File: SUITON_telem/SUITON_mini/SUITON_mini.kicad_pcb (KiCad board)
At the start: 2 copper layers, 81 parts, among them J3 USB_C_Receptacle_USB2.0_16P, Q2 AO3407A, Q3 BSS138, Q4 BSS138, Q5 BSS138, U1 W25Q128JVPIQ, U10 LSM6DSV320XTR, U11 USBLC6-2P6, U12 TPS1H200AQDGNRQ1, U13 AP2112K-3.3TRG1, U14 TPS1H200AQDGNRQ1, U2 TPS63070RNMR, U4 AP2112K-3.3TRG1, U5 STM32F405RGT6, U6 E22-900MM22S, U7 ISM330DHCXTR, U8 SAM-M10Q-00B, U9 BMP581, X1 ABM3B-8.000MHZ-10-1UT

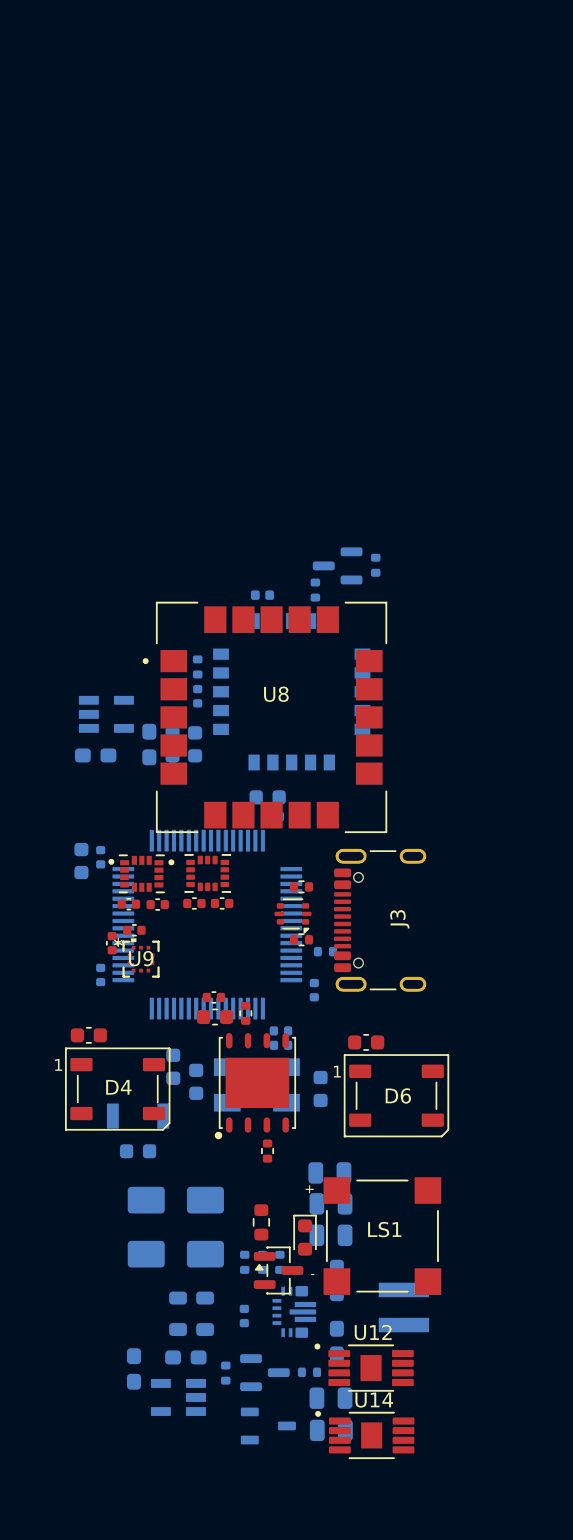
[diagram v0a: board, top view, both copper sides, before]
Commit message: Shape
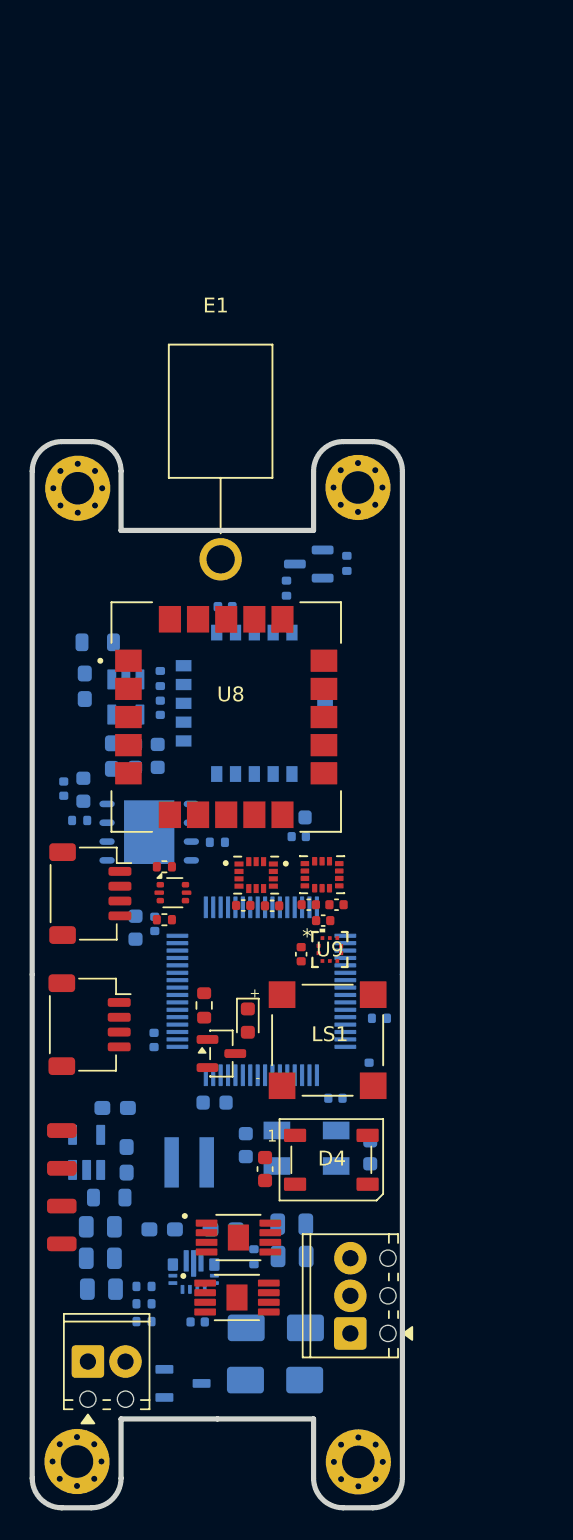
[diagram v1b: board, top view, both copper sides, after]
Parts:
- removed C21, C36: 100nF, Capacitor_SMD:C_0603_1608Metric
- removed C35: 1uF, Capacitor_SMD:C_0402_1005Metric
- removed D3, D7: SS34, Diode_SMD:D_SMA
- removed D6: WS2812B, LED_SMD:LED_WS2812B_PLCC4_5.0x5.0mm_P3.2mm
- removed J3: USB_C_Receptacle_USB2.0_16P, Connector_USB:USB_C_Receptacle_GCT_USB4105-xx-A_16P_TopMnt_Horizontal
- removed Q5: BSS138, Package_TO_SOT_SMD:SOT-23
- removed R2: 100kΩ, Resistor_SMD:R_0402_1005Metric
- removed S3: B3U-1000P, B3U-1000P:SW_B3U-1000P
- added D8: SS34, Diode_SMD:D_SMA, B.Cu at (145.4, 135.4)
- added D9: SS34, Diode_SMD:D_SMA, B.Cu at (145.5, 131.9)
- added E1: ANT-868-JJB-RA, ANT-868-JJB-RA:XDCR_ANT-868-JJB-RA, F.Cu at (141.8, 80.0)
- added H1: MountingHole_Pad, MountingHole:MountingHole_2.2mm_M2_Pad_Via, F.Cu at (132.1, 75.2)
- added H2: MountingHole_Pad, MountingHole:MountingHole_2.2mm_M2_Pad_Via, F.Cu at (151.1, 75.1)
- added H3: MountingHole_Pad, MountingHole:MountingHole_2.2mm_M2_Pad_Via, F.Cu at (132.1, 140.9)
- added H4: MountingHole_Pad, MountingHole:MountingHole_2.2mm_M2_Pad_Via, F.Cu at (151.1, 140.9)
- added J1: Conn_01x02_Pin, TerminalBlock_Phoenix:TerminalBlock_Phoenix_MPT-0,5-2-2.54_1x02_P2.54mm_Horizontal, F.Cu at (132.8, 134.2)
- added J2: Conn_01x04_Pin, Connector_JST:JST_SH_SM04B-SRSS-TB_1x04-1MP_P1.00mm_Horizontal, F.Cu at (133.0, 102.5)
- added J2: Conn_01x04_Pin, Connector_JST:JST_SH_SM04B-SRSS-TB_1x04-1MP_P1.00mm_Horizontal, F.Cu at (132.9, 111.4)
- added J5: Conn_01x03_Pin, TerminalBlock_Phoenix:TerminalBlock_Phoenix_MPT-0,5-3-2.54_1x03_P2.54mm_Horizontal, F.Cu at (150.5, 132.2)
- added J6: Conn_01x01_Pin, Connector_Wire:SolderWirePad_1x01_SMD_1x2mm, F.Cu at (131.1, 126.2)
- added J7: Conn_01x01_Pin, Connector_Wire:SolderWirePad_1x01_SMD_1x2mm, F.Cu at (131.1, 123.7)
- added J8: Conn_01x01_Pin, Connector_Wire:SolderWirePad_1x01_SMD_1x2mm, F.Cu at (131.1, 121.1)
- added J9: Conn_01x01_Pin, Connector_Wire:SolderWirePad_1x01_SMD_1x2mm, F.Cu at (131.1, 118.6)
- C22, C23, R30, R31, U1: moved to B.Cu
- moved FB2 45.7 mm to (133.5, 85.6), turned to 0 degrees
- moved R30 21.1 mm to (141.6, 99.1), turned to 180 degrees
- moved U1 18.4 mm to (136.9, 98.4), turned to 180 degrees
- moved C23 17.7 mm to (132.5, 95.5), turned to -90 degrees
- moved U4 17.7 mm to (132.7, 120.0), turned to 90 degrees
- moved C11 17.7 mm to (134.7, 117.0), turned to 0 degrees
- moved L3 17.5 mm to (139.7, 120.7), turned to 0 degrees
- moved C22 17.4 mm to (131.2, 95.5), turned to -90 degrees
- moved C8 17.3 mm to (133.7, 129.3), turned to 180 degrees
- moved R31 17.2 mm to (132.3, 97.6), turned to 0 degrees
- moved U14 16.1 mm to (143.0, 125.8)
- moved C7 16.0 mm to (133.7, 127.2), turned to 180 degrees
- moved C6 15.6 mm to (133.7, 125.0), turned to 180 degrees
- moved D4 15.2 mm to (149.2, 120.5)
- moved D5 15.2 mm to (143.6, 111.1)
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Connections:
- net /MCU/USB_DM renamed /MCU/USB_D-
- net /MCU/USB_DP renamed /MCU/USB_D+
- C1 pad 1: VCC -> Net-(D8-K)
- C2 pad 1: VCC -> Net-(D8-K)
- C3 pad 1: VCC -> Net-(D8-K)
- C5 pad 1: Net-(D3-A) -> +5V
- C6 pad 1: Net-(D3-A) -> +5V
- C7 pad 1: Net-(D3-A) -> +5V
- C8 pad 1: Net-(D3-A) -> +5V
- D4 pad 2: Net-(D4-DOUT) -> unconnected-(D4-DOUT-Pad2)
- R4 pad 2: VCC -> Net-(D8-K)
- R5 pad 1: Net-(D3-A) -> +5V
- R6 pad 1: Net-(D3-A) -> +5V
- U2 pad 12_13: VCC -> Net-(D8-K)
- U2 pad 7_8: Net-(D3-A) -> +5V
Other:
- board outline added: 25 x 72 mm

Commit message: Suiton mini
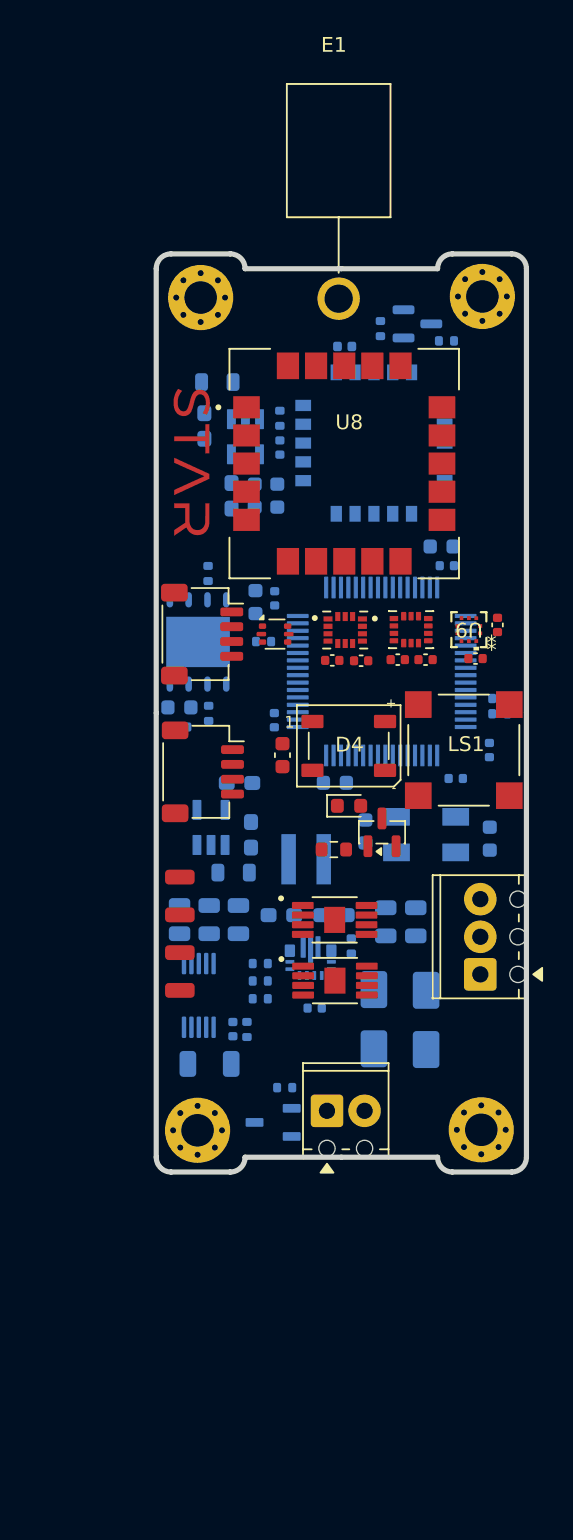
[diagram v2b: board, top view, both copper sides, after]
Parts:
- removed the J2 at (133.0, 102.5)
- removed the J2 at (132.9, 111.4)
- removed R23, R24: 5k1, Resistor_SMD:R_0402_1005Metric
- added C9: 100nF, Capacitor_SMD:C_0402_1005Metric, B.Cu at (142.6, 111.7)
- added G***: LOGO, star:logo_satr, F.Cu at (139.8, 73.4)
- added J2: Conn_01x04_Pin, Connector_JST:JST_SH_SM04B-SRSS-TB_1x04-1MP_P1.00mm_Horizontal, F.Cu at (140.6, 94.3)
- added J2: Conn_01x04_Pin, Connector_JST:JST_SH_SM04B-SRSS-TB_1x04-1MP_P1.00mm_Horizontal, F.Cu at (140.5, 85.0)
- added R1: 20m, Resistor_SMD:R_1206_3216Metric, B.Cu at (141.0, 114.0)
- added R37: 10kΩ, Resistor_SMD:R_0402_1005Metric, B.Cu at (144.7, 85.5)
- added R38: 10kΩ, Resistor_SMD:R_0402_1005Metric, B.Cu at (160.6, 90.4)
- added R8: 10k, Resistor_SMD:R_0402_1005Metric, B.Cu at (143.6, 111.7)
- added R9: 10k, Resistor_SMD:R_0402_1005Metric, B.Cu at (146.1, 115.7)
- added U3: INA226, Package_SO:TSSOP-10_3x3mm_P0.5mm, B.Cu at (140.3, 109.4)
- moved C20 28.0 mm to (145.9, 93.2)
- moved D4 28.0 mm to (150.4, 92.6)
- moved C16 25.9 mm to (160.5, 84.4), turned to -90 degrees
- moved J5 25.8 mm to (159.3, 108.0)
- moved C8 25.5 mm to (139.0, 104.3), turned to 90 degrees
- moved D8 25.3 mm to (152.1, 111.0), turned to -90 degrees
- moved C1 24.1 mm to (155.0, 104.5), turned to 90 degrees
- moved C7 24.0 mm to (141.0, 104.3), turned to 90 degrees
- moved H4 23.9 mm to (159.4, 118.5)
- moved H3 23.8 mm to (140.2, 118.5)
- moved U9 23.6 mm to (158.5, 84.7), turned to 180 degrees
- moved C11 23.5 mm to (143.0, 95.1)
- moved C10 23.5 mm to (143.8, 98.6)
- moved FB1 23.5 mm to (142.7, 101.1)
- moved U4 23.5 mm to (141.1, 98.1)
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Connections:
- D8 pad 2: VCC -> Net-(D8-A)
- U5 pad 15: unconnected-(U5-PA1/USART2_RTS-Pad15) -> Alert
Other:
- board size 25 x 72 mm -> 25 x 62 mm
